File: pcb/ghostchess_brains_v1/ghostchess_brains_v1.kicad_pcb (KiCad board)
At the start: 2 copper layers, 150 x 50 mm, 15 parts, among them J1 ISP, SW1 SW_Push, SW2 SW_Push, SW3 SW_Push, U1 ATmega644PA-P, Y1 11.0592MHz

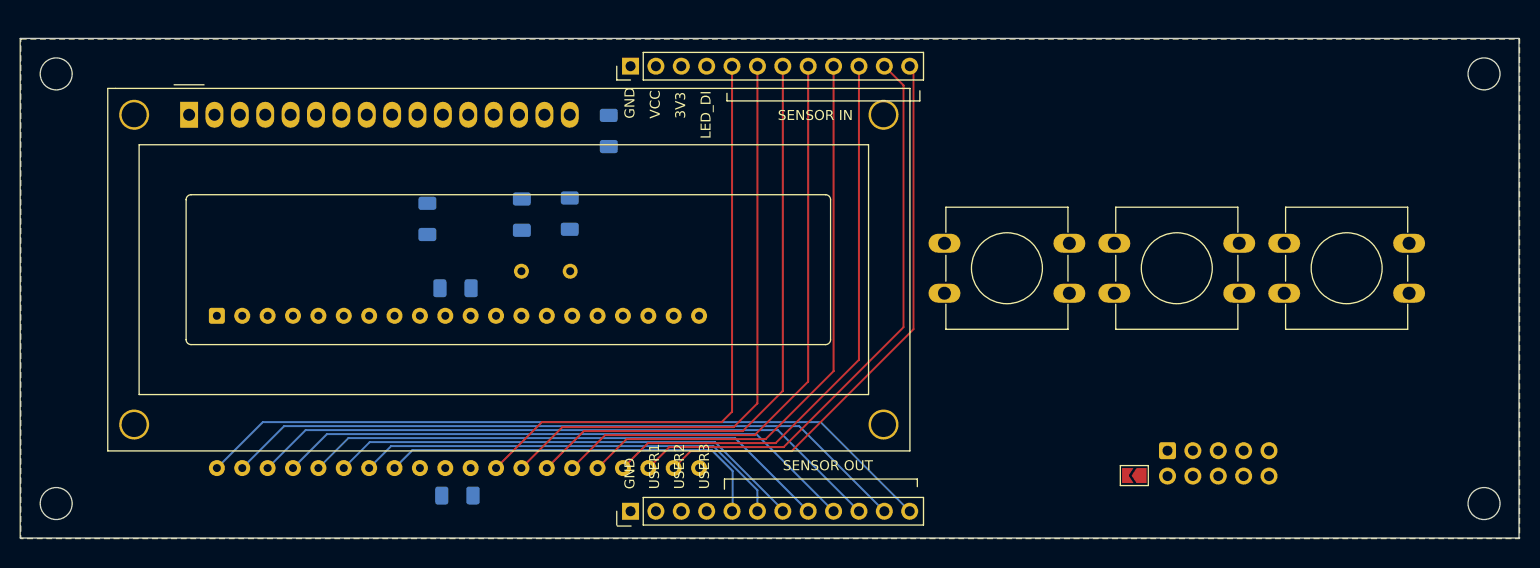
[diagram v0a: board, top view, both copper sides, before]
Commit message: brains v1 board
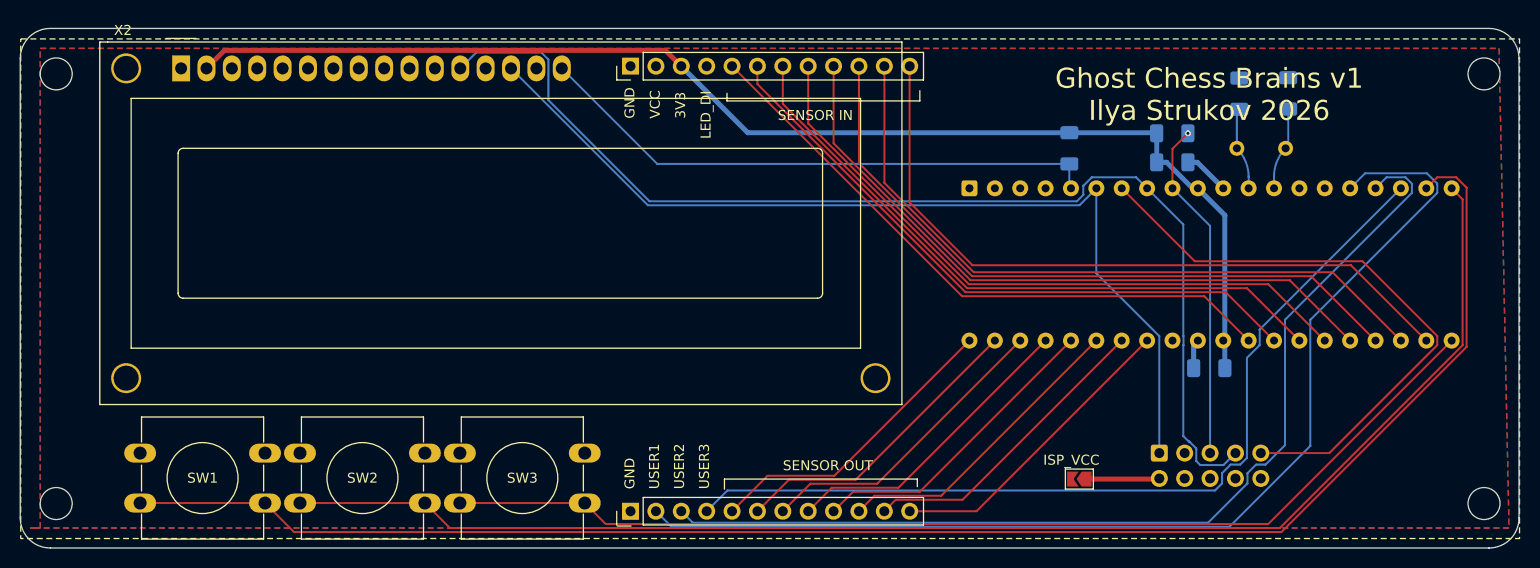
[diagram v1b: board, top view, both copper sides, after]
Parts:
- X2: footprint Display:WC1602A -> ghostchess:WC1602A_3Hole
- moved SW3 85.1 mm to (94.0, 91.5)
- moved SW2 84.2 mm to (78.0, 91.5)
- moved SW1 83.2 mm to (62.0, 91.5)
- moved C3 78.9 mm to (165.3, 62.4), turned to 0 degrees
- moved U1 76.4 mm to (145.0, 65.0)
- moved C4 75.9 mm to (169.0, 83.0), turned to 180 degrees
- moved R1 75.0 mm to (165.3, 59.5), turned to 0 degrees
- moved C1 72.9 mm to (176.9, 55.5)
- moved C2 72.8 mm to (172.0, 55.5)
- moved Y1 72.6 mm to (171.8, 61.0)
- moved R2 46.1 mm to (155.0, 61.0), turned to -90 degrees
- moved JP1 5.51 mm to (156.0, 94.1)
- moved X2 4.71 mm to (66.1, 53.0)
- moved J1 0.85 mm to (164.0, 91.5)
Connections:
- U1 pad 33: /SENSOR_OUT_1 -> /SENSOR_OUT_8
- U1 pad 34: /SENSOR_OUT_2 -> /SENSOR_OUT_7
- U1 pad 35: /SENSOR_OUT_3 -> /SENSOR_OUT_6
- U1 pad 36: /SENSOR_OUT_4 -> /SENSOR_OUT_5
- U1 pad 37: /SENSOR_OUT_5 -> /SENSOR_OUT_4
- U1 pad 38: /SENSOR_OUT_6 -> /SENSOR_OUT_3
- U1 pad 39: /SENSOR_OUT_7 -> /SENSOR_OUT_2
- U1 pad 40: /SENSOR_OUT_8 -> /SENSOR_OUT_1
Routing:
- net /BTN1: track 0.00 -> 162.5 mm
- net /BTN2: track 0.00 -> 141.1 mm
- net VCC: track 0.00 -> 126.5 mm
- net /OLED_SCL: track 0.00 -> 113.9 mm
- net /USER1: track 0.00 -> 110.8 mm
- net /BTN3: track 0.00 -> 107.7 mm
- net /USER2: track 0.00 -> 100.5 mm
- net /MOSI: track 0.00 -> 94.1 mm
- net /USER3: track 0.00 -> 90.2 mm
- net /MISO: track 0.00 -> 60.8 mm
- net /OLED_CS: track 0.00 -> 57.3 mm
- net /SENSOR_OUT_8: track 74.9 -> 30.8 mm
- net /SENSOR_OUT_7: track 69.5 -> 30.8 mm
- net /~{RESET}: track 0.00 -> 34.2 mm, vias 0 -> 1
- net /SENSOR_OUT_6: track 64.1 -> 30.8 mm
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- added copper zone on B.Cu, net GND
- added copper zone on F.Cu, net GND
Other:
- board size 150 x 50 mm -> 150 x 52 mm
- board text added: "Ghost Chess Brains v1 Ilya Strukov 2026"
